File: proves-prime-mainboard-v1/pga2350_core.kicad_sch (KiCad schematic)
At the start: 19 parts, among them J6 USB_C_Receptacle_USB2.0_16P, SW1 KMR2, SW2 KMR2, SW4 SW_SPDT

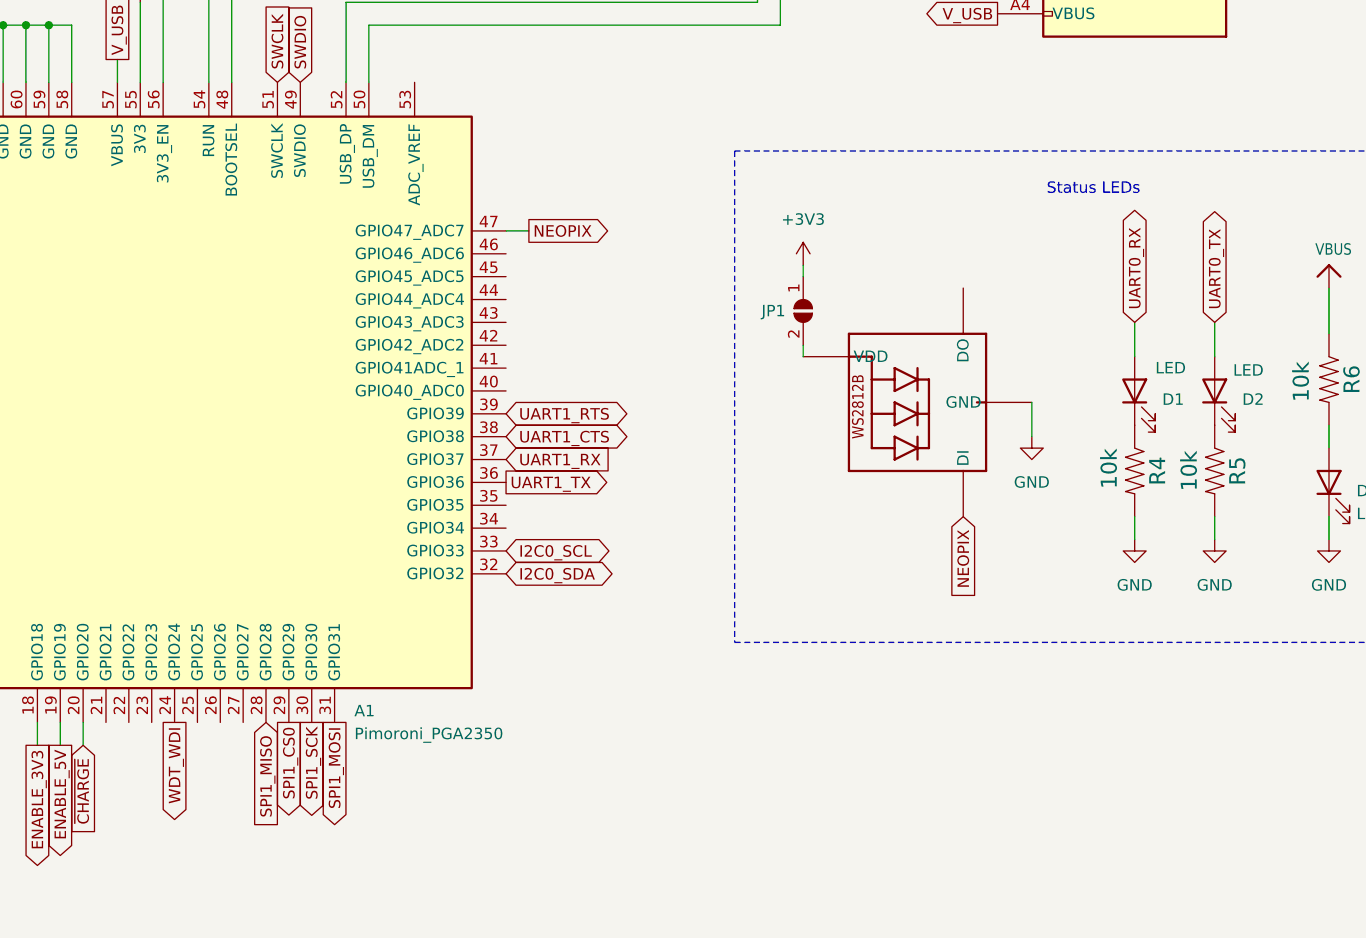
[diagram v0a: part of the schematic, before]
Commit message: Created MVS Sheet
Minimum Viable Satellite
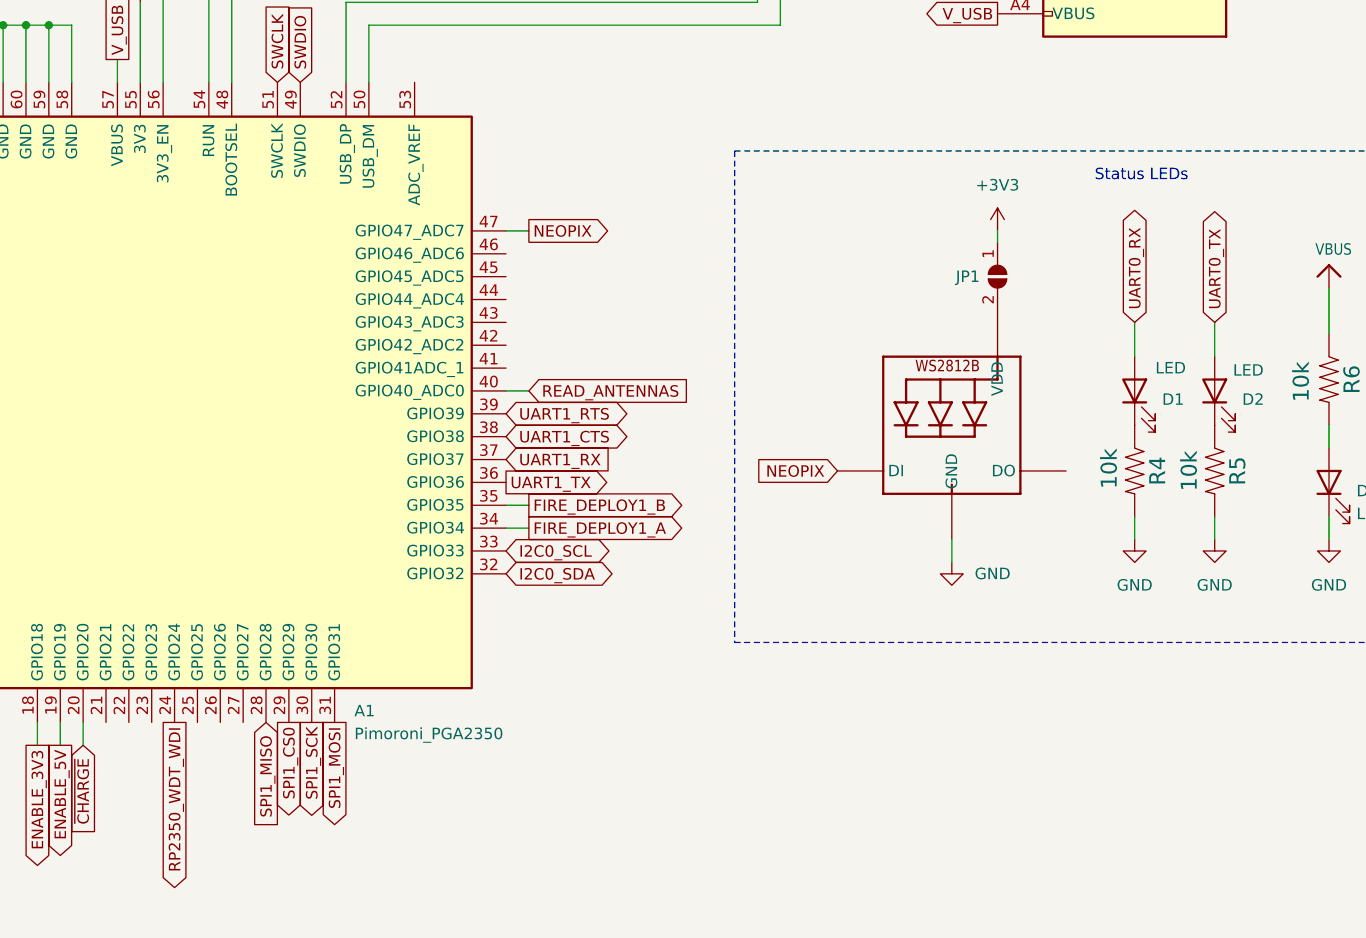
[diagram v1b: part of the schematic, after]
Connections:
- net FIRE_DEPLOY1_A: now reaches A1.34 (GPIO34)
- net FIRE_DEPLOY1_B: now reaches A1.35 (GPIO35)
- net READ_ANTENNAS: now reaches A1.40 (GPIO40_ADC0)
- net WDT_WDI renamed RP2350_WDT_WDI
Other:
- moved on the sheet: JP1
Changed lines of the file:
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@@
 	(wire
 		(pts
-			(xy 201.93 95.25) (xy 201.93 96.52)
+			(xy 125.73 63.5) (xy 125.73 66.04)
 		)
 		(stroke
@@
 	(wire
 		(pts
-			(xy 125.73 63.5) (xy 125.73 66.04)
+			(xy 163.83 34.29) (xy 163.83 44.45)
 		)
 		(stroke
@@
 	(wire
 		(pts
-			(xy 163.83 34.29) (xy 163.83 44.45)
+			(xy 223.52 83.82) (xy 223.52 82.55)
 		)
 		(stroke
@@
 		)
 	)
+	(wire
+		(pts
+			(xy 218.44 119.38) (xy 218.44 116.84)
+		)
+		(stroke
+			(width 0)
+			(type default)
+		)
+	)
 	(polyline
 		(pts
@@
 	(wire
 		(pts
-			(xy 201.93 86.36) (xy 201.93 87.63)
+			(xy 163.83 44.45) (xy 163.83 45.72)
 		)
 		(stroke
@@
 	(wire
 		(pts
-			(xy 163.83 44.45) (xy 163.83 45.72)
+			(xy 168.91 115.57) (xy 171.45 115.57)
 		)
 		(stroke
@@
 	(wire
 		(pts
+			(xy 168.91 113.03) (xy 171.45 113.03)
+		)
+		(stroke
+			(width 0)
+			(type default)
+		)
+	)
+	(wire
+		(pts
 			(xy 199.39 59.69) (xy 199.39 43.18)
 		)
@@
 	(wire
 		(pts
+			(xy 168.91 100.33) (xy 171.45 100.33)
+		)
+		(stroke
+			(width 0)
+			(type default)
+		)
+	)
+	(wire
+		(pts
 			(xy 128.27 57.15) (xy 128.27 66.04)
 		)
@@
 		)
 	)
-	(wire
-		(pts
-			(xy 227.33 105.41) (xy 227.33 101.6)
-		)
-		(stroke
-			(width 0)
-			(type default)
-		)
-	)
 	(text "Check if USBBOOT\nNeeds Pull Up"
 		(exclude_from_sim no)
@@
 	(text "Status LEDs"
 		(exclude_from_sim no)
-		(at 234.188 77.978 0)
+		(at 239.522 76.454 0)
 		(effects
 			(font
@@
 		)
 	)
-	(global_label "WDT_WDI"
+	(global_label "RP2350_WDT_WDI"
 		(shape output)
 		(at 132.08 137.16 270)
@@
 		)
 		(property "Intersheetrefs" "${INTERSHEET_REFS}"
-			(at 132.08 148.128 90)
+			(at 132.08 156.4736 90)
 			(effects
 				(font
@@
 		)
 	)
+	(global_label "FIRE_DEPLOY1_B"
+		(shape output)
+		(at 171.45 113.03 0)
+		(fields_autoplaced yes)
+		(effects
+			(font
+				(size 1.27 1.27)
+			)
+			(justify left)
+		)
+		(property "Intersheetrefs" "${INTERSHEET_REFS}"
+			(at 190.0985 113.03 0)
+			(effects
+				(font
+					(size 1.27 1.27)
+				)
+				(justify left)
+				(hide yes)
+			)
+		)
+	)
 	(global_label "I2C0_SDA"
 		(shape bidirectional)
@@
 		)
 	)
+	(global_label "READ_ANTENNAS"
+		(shape input)
+		(at 171.45 100.33 0)
+		(fields_autoplaced yes)
+		(effects
+			(font
+				(size 1.27 1.27)
+			)
+			(justify left)
+		)
+		(property "Intersheetrefs" "${INTERSHEET_REFS}"
+			(at 189.6752 100.33 0)
+			(effects
+				(font
+					(size 1.27 1.27)
+				)
+				(justify left)
+				(hide yes)
+			)
+		)
+	)
 	(global_label "I2C1_SDA"
 		(shape bidirectional)
@@
 		)
 	)
+	(global_label "FIRE_DEPLOY1_A"
+		(shape output)
+		(at 171.45 115.57 0)
+		(fields_autoplaced yes)
+		(effects
+			(font
+				(size 1.27 1.27)
+			)
+			(justify left)
+		)
+		(property "Intersheetrefs" "${INTERSHEET_REFS}"
+			(at 189.9171 115.57 0)
+			(effects
+				(font
+					(size 1.27 1.27)
+				)
+				(justify left)
+				(hide yes)
+			)
+		)
+	)
 	(global_label "SPI0_MISO"
 		(shape input)
@@
 	(global_label "NEOPIX"
 		(shape input)
-		(at 219.71 114.3 270)
+		(at 205.74 109.22 180)
 		(fields_autoplaced yes)
 		(effects
@@
 		)
 		(property "Intersheetrefs" "${INTERSHEET_REFS}"
-			(at 219.71 124.1795 90)
+			(at 195.8605 109.22 0)
 			(effects
 				(font
@@
 	(symbol
 		(lib_id "power:GND")
-		(at 227.33 105.41 0)
+		(at 218.44 119.38 0)
 		(unit 1)
 		(exclude_from_sim no)
@@
 		(fields_autoplaced yes)
 		(property "Reference" "#PWR022"
-			(at 227.33 111.76 0)
+			(at 218.44 125.73 0)
 			(effects
 				(font
@@
 		)
 		(property "Value" "GND"
-			(at 227.33 110.49 0)
+			(at 220.98 120.6499 0)
 			(effects
 				(font
 					(size 1.27 1.27)
 				)
+				(justify left)
 			)
 		)
 		(property "Footprint" ""
-			(at 227.33 105.41 0)
+			(at 218.44 119.38 0)
 			(effects
 				(font
@@
 		)
 		(property "Datasheet" ""
-			(at 227.33 105.41 0)
+			(at 218.44 119.38 0)
 			(effects
 				(font
@@
 		)
 		(property "Description" ""
-			(at 227.33 105.41 0)
+			(at 218.44 119.38 0)
 			(effects
 				(font
@@
 	(symbol
 		(lib_id "Jumper:SolderJumper_2_Open")
-		(at 201.93 91.44 270)
+		(at 223.52 87.63 270)
 		(unit 1)
 		(exclude_from_sim no)
@@
 		(dnp no)
 		(property "Reference" "JP1"
-			(at 198.628 91.44 90)
+			(at 220.218 87.63 90)
 			(effects
 				(font
@@
 		)
 		(property "Value" "SolderJumper_2_Open"
-			(at 215.9 91.44 90)
+			(at 237.49 87.63 90)
 			(effects
 				(font
@@
 		)
 		(property "Footprint" "Jumper:SolderJumper-2_P1.3mm_Open_RoundedPad1.0x1.5mm"
-			(at 201.93 91.44 0)
+			(at 223.52 87.63 0)
 			(effects
 				(font
@@
 		)
 		(property "Datasheet" "~"
-			(at 201.93 91.44 0)
+			(at 223.52 87.63 0)
 			(effects
 				(font
@@
 		)
 		(property "Description" ""
-			(at 201.93 91.44 0)
+			(at 223.52 87.63 0)
 			(effects
 				(font
@@
 	(symbol
 		(lib_id "Adafruit ItsyBitsy RP2040-eagle-import:WS2812B_SK6805_1515")
-		(at 217.17 101.6 90)
+		(at 218.44 106.68 0)
 		(unit 1)
 		(exclude_from_sim no)
@@
 		(dnp no)
 		(property "Reference" "LED1"
-			(at 217.17 101.6 0)
+			(at 218.44 106.68 0)
 			(effects
 				(font
@@
 		)
 		(property "Value" "WS2812B_SK6812_1515"
-			(at 217.17 101.6 0)
+			(at 218.44 106.68 0)
 			(effects
 				(font
@@
 		)
 		(property "Footprint" "LED_SMD:LED_WS2812B_PLCC4_5.0x5.0mm_P3.2mm"
-			(at 217.17 101.6 0)
+			(at 218.44 106.68 0)
 			(effects
 				(font
@@
 		)
 		(property "Datasheet" ""
-			(at 217.17 101.6 0)
+			(at 218.44 106.68 0)
 			(effects
 				(font
@@
 		)
 		(property "Description" ""
-			(at 217.17 101.6 0)
+			(at 218.44 106.68 0)
 			(effects
 				(font
@@
 		(lib_name "+3V3_2")
 		(lib_id "power:+3V3")
-		(at 201.93 86.36 0)
+		(at 223.52 82.55 0)
 		(unit 1)
 		(exclude_from_sim no)
@@
 		(fields_autoplaced yes)
 		(property "Reference" "#PWR020"
-			(at 201.93 90.17 0)
+			(at 223.52 86.36 0)
 			(effects
 				(font
@@
 		)
 		(property "Value" "+3V3"
-			(at 201.93 81.28 0)
+			(at 223.52 77.47 0)
 			(effects
 				(font
@@
 		)
 		(property "Footprint" ""
-			(at 201.93 86.36 0)
+			(at 223.52 82.55 0)
 			(effects
 				(font
@@
 		)
 		(property "Datasheet" ""
-			(at 201.93 86.36 0)
+			(at 223.52 82.55 0)
 			(effects
 				(font
@@
 		)
 		(property "Description" "Power symbol creates a global label with name \"+3V3\""
-			(at 201.93 86.36 0)
+			(at 223.52 82.55 0)
 			(effects
 				(font
